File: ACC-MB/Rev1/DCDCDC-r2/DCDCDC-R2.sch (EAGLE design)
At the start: 21 parts, among them X2 5566-4

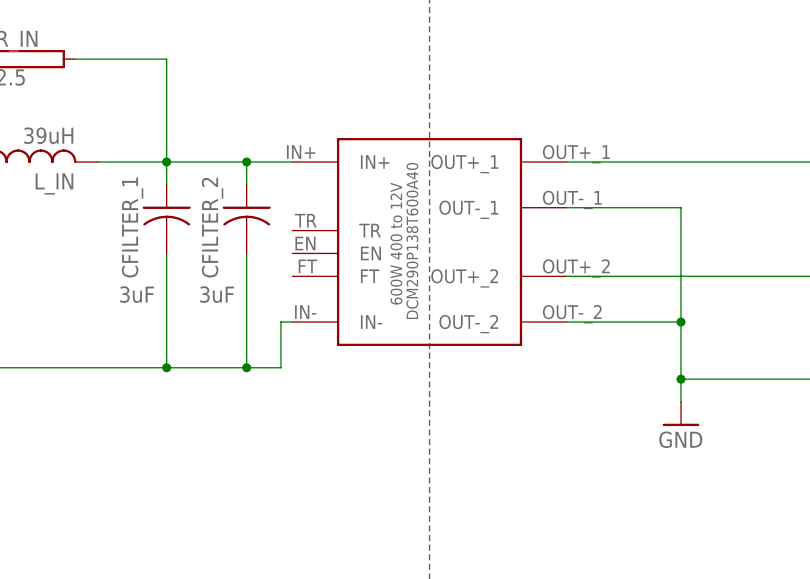
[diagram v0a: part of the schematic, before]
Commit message: update
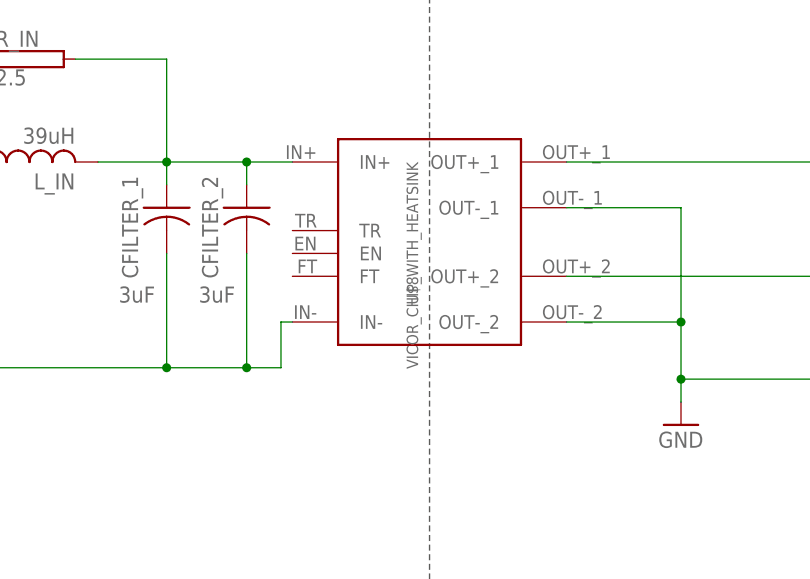
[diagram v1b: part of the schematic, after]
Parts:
- U$8: value 600W 400 to 12V -> VICOR_CHIP_WITH_HEATSINK
- renumbered DCM290P138T600A40 to U$8
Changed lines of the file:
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@@
 <parts>
 <part name="FRAME1" library="ACC-MB-R0" library_urn="urn:adsk.eagle:library:13324935" deviceset="A3L-LOC" device=""/>
-<part name="DCM290P138T600A40" library="ACC-MB-R0" library_urn="urn:adsk.eagle:library:13324935" deviceset="VICOR_CHIP_WITH_HEATSINK" device="" package3d_urn="urn:adsk.eagle:package:13209498/1" value="600W 400 to 12V"/>
 <part name="P+2" library="ACC-MB-R0" library_urn="urn:adsk.eagle:library:13324935" deviceset="V+" device=""/>
 <part name="P-1" library="ACC-MB-R0" library_urn="urn:adsk.eagle:library:13324935" deviceset="V-" device=""/>
@@
 <part name="P+5" library="ACC-MB-R0" library_urn="urn:adsk.eagle:library:13208985" deviceset="+12V" device=""/>
 <part name="GND1" library="ACC-MB-R0" library_urn="urn:adsk.eagle:library:13208985" deviceset="GND" device=""/>
+<part name="U$8" library="ACC-MB-R0" library_urn="urn:adsk.eagle:library:13208985" deviceset="VICOR_CHIP_WITH_HEATSINK" device="" package3d_urn="urn:adsk.eagle:package:13209498/2"/>
 </parts>
 <sheets>
@@
 <attribute name="SHEET" x="357.505" y="5.08" size="2.54" layer="94"/>
 </instance>
-<instance part="DCM290P138T600A40" gate="G$1" x="105.41" y="219.71" smashed="yes" rot="R270">
-<attribute name="VALUE" x="111.252" y="217.424" size="1.27" layer="96" rot="R270"/>
-<attribute name="NAME" x="113.03" y="219.71" size="1.27" layer="95" rot="R270"/>
-</instance>
 <instance part="P+2" gate="1" x="27.94" y="229.87" smashed="yes">
 <attribute name="VALUE" x="25.4" y="227.33" size="1.778" layer="96" rot="R90"/>
@@
 <instance part="P+5" gate="1" x="19.05" y="139.7"/>
 <instance part="GND1" gate="1" x="19.05" y="107.95"/>
+<instance part="U$8" gate="G$1" x="105.41" y="219.71" rot="R270"/>
 </instances>
 <busses>
@@
 </segment>
 <segment>
-<pinref part="DCM290P138T600A40" gate="G$1" pin="OUT-_1"/>
 <wire x1="130.81" y1="214.63" x2="143.51" y2="214.63" width="0.1524" layer="91"/>
 <wire x1="143.51" y1="214.63" x2="143.51" y2="201.93" width="0.1524" layer="91"/>
-<pinref part="DCM290P138T600A40" gate="G$1" pin="OUT-_2"/>
 <wire x1="143.51" y1="201.93" x2="143.51" y2="195.58" width="0.1524" layer="91"/>
 <wire x1="143.51" y1="195.58" x2="143.51" y2="193.04" width="0.1524" layer="91"/>
@@
 <wire x1="162.56" y1="195.58" x2="143.51" y2="195.58" width="0.1524" layer="91"/>
 <junction x="143.51" y="195.58"/>
+<pinref part="U$8" gate="G$1" pin="OUT-_1"/>
+<pinref part="U$8" gate="G$1" pin="OUT-_2"/>
 </segment>
 <segment>
@@
 <pinref part="CFILTER_2" gate="G$1" pin="2"/>
 <wire x1="95.25" y1="209.55" x2="95.25" y2="196.85" width="0.1524" layer="91"/>
-<pinref part="DCM290P138T600A40" gate="G$1" pin="IN-"/>
 <wire x1="100.33" y1="201.93" x2="99.06" y2="201.93" width="0.1524" layer="91"/>
 <wire x1="99.06" y1="201.93" x2="99.06" y2="196.85" width="0.1524" layer="91"/>
 <wire x1="99.06" y1="196.85" x2="95.25" y2="196.85" width="0.1524" layer="91"/>
 <junction x="95.25" y="196.85"/>
+<pinref part="U$8" gate="G$1" pin="IN-"/>
 </segment>
 <segment>
@@
 <segment>
 <pinref part="L_IN" gate="G$1" pin="2"/>
-<pinref part="DCM290P138T600A40" gate="G$1" pin="IN+"/>
 <wire x1="78.74" y1="219.71" x2="86.36" y2="219.71" width="0.1524" layer="91"/>
 <pinref part="CFILTER_1" gate="G$1" pin="1"/>
@@
 <wire x1="76.2" y1="231.14" x2="86.36" y2="231.14" width="0.1524" layer="91"/>
 <wire x1="86.36" y1="231.14" x2="86.36" y2="219.71" width="0.1524" layer="91"/>
+<pinref part="U$8" gate="G$1" pin="IN+"/>
 </segment>
 </net>
@@
 <net name="DCDC_OUT" class="1">
 <segment>
-<pinref part="DCM290P138T600A40" gate="G$1" pin="OUT+_1"/>
 <wire x1="130.81" y1="219.71" x2="162.56" y2="219.71" width="0.1524" layer="91"/>
-<pinref part="DCM290P138T600A40" gate="G$1" pin="OUT+_2"/>
 <wire x1="130.81" y1="207.01" x2="162.56" y2="207.01" width="0.1524" layer="91"/>
 <wire x1="162.56" y1="207.01" x2="162.56" y2="219.71" width="0.1524" layer="91"/>
@@
 <wire x1="162.56" y1="205.74" x2="162.56" y2="207.01" width="0.1524" layer="91"/>
 <junction x="162.56" y="207.01"/>
-</segment>
-<segment>
+<pinref part="U$8" gate="G$1" pin="OUT+_1"/>
+<pinref part="U$8" gate="G$1" pin="OUT+_2"/>
+</segment>
+<segment>
